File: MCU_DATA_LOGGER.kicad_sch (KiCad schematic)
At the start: 25 parts, among them U1 DS1337S+, U2 24LC1025, U3 24LC1025, U4 ATMEGA328P-AU, Y1 32.768 KHz, Y2 16 MHz

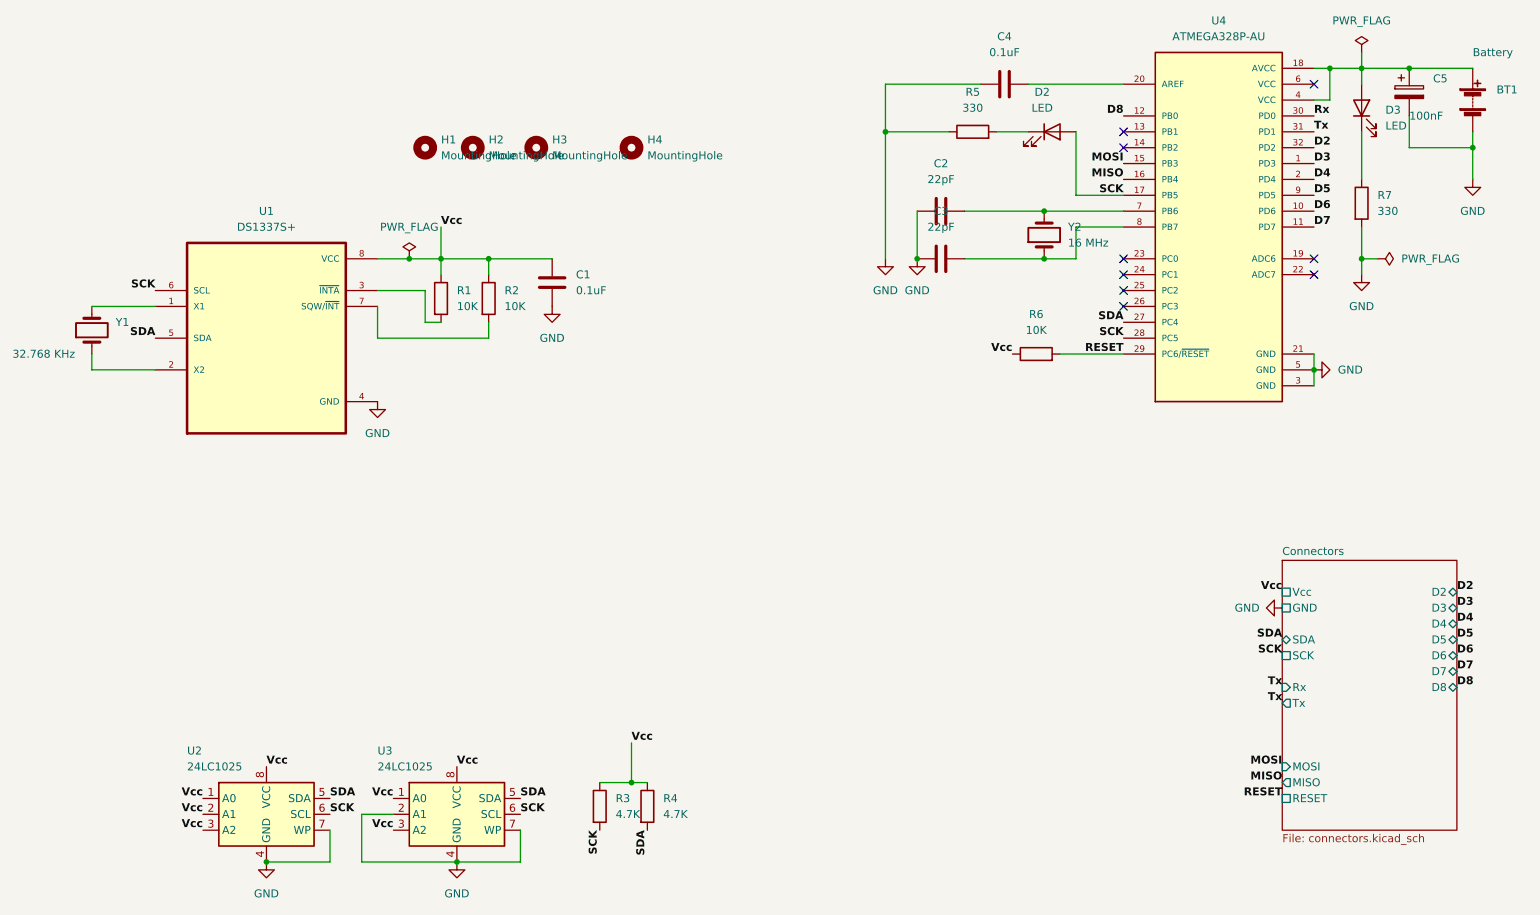
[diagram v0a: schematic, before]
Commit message: Completed schematic
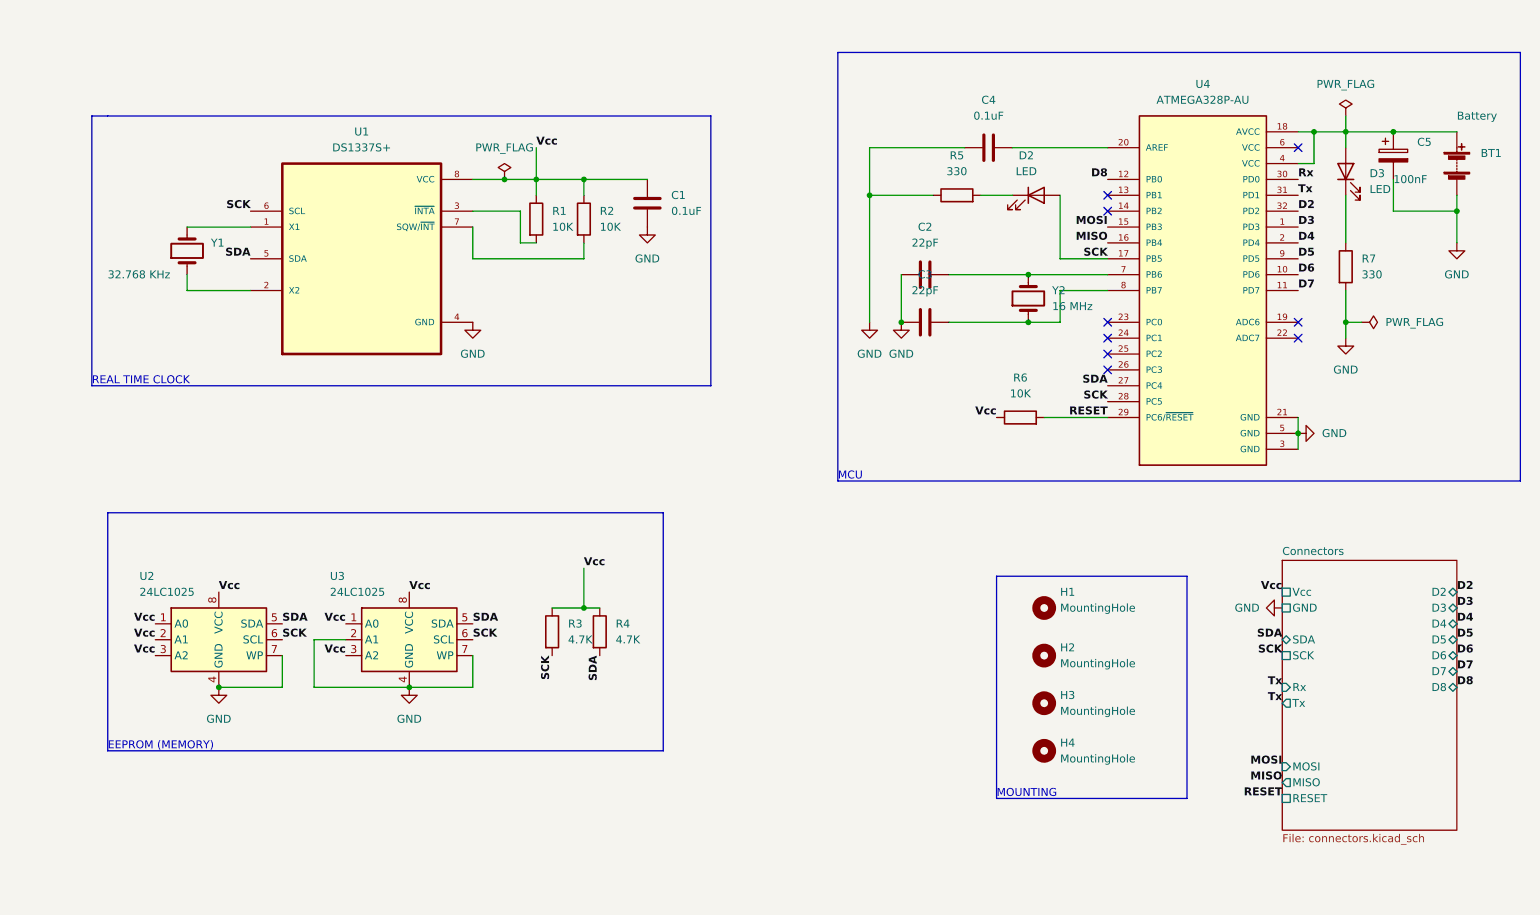
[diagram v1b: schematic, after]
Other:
- note added: "EEPROM (MEMORY)"
- note added: "MCU"
- note added: "MOUNTING"
- note added: "REAL TIME CLOCK"
- moved on the sheet: BT1, C1, C2, C3, C4, C5, D2, D3, H1, H2, H3, H4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
